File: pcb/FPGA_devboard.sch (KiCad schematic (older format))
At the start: 2 parts, among them X3 AC7020, X4 Conn_02x05_Odd_Even

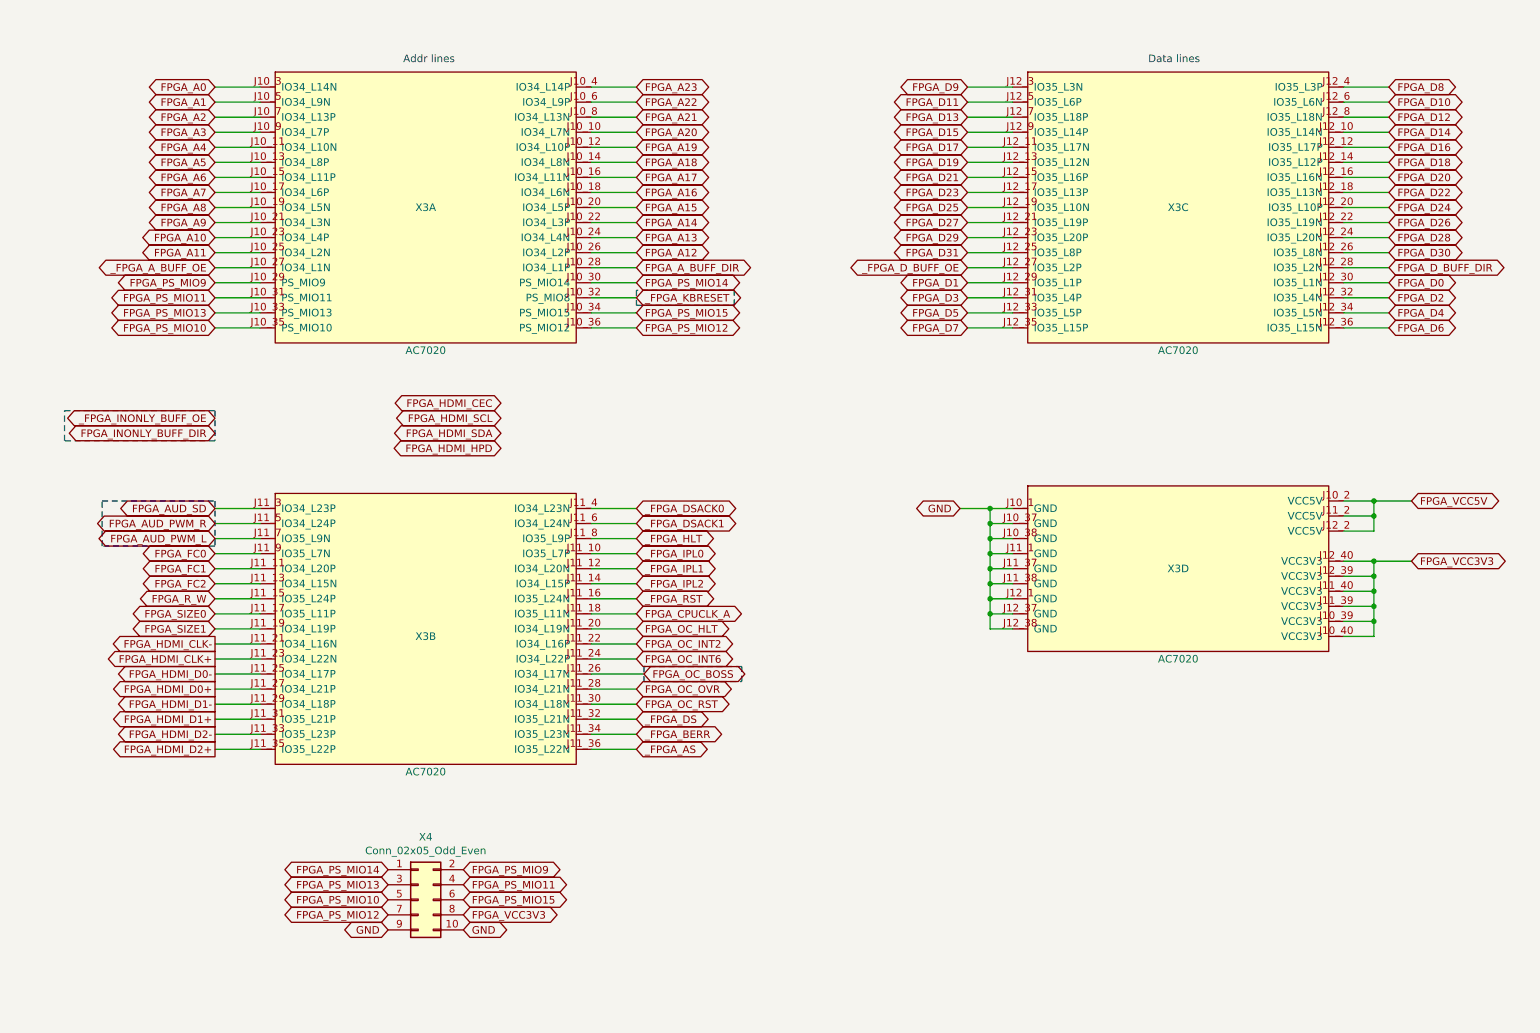
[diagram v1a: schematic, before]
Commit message: time to stop for today
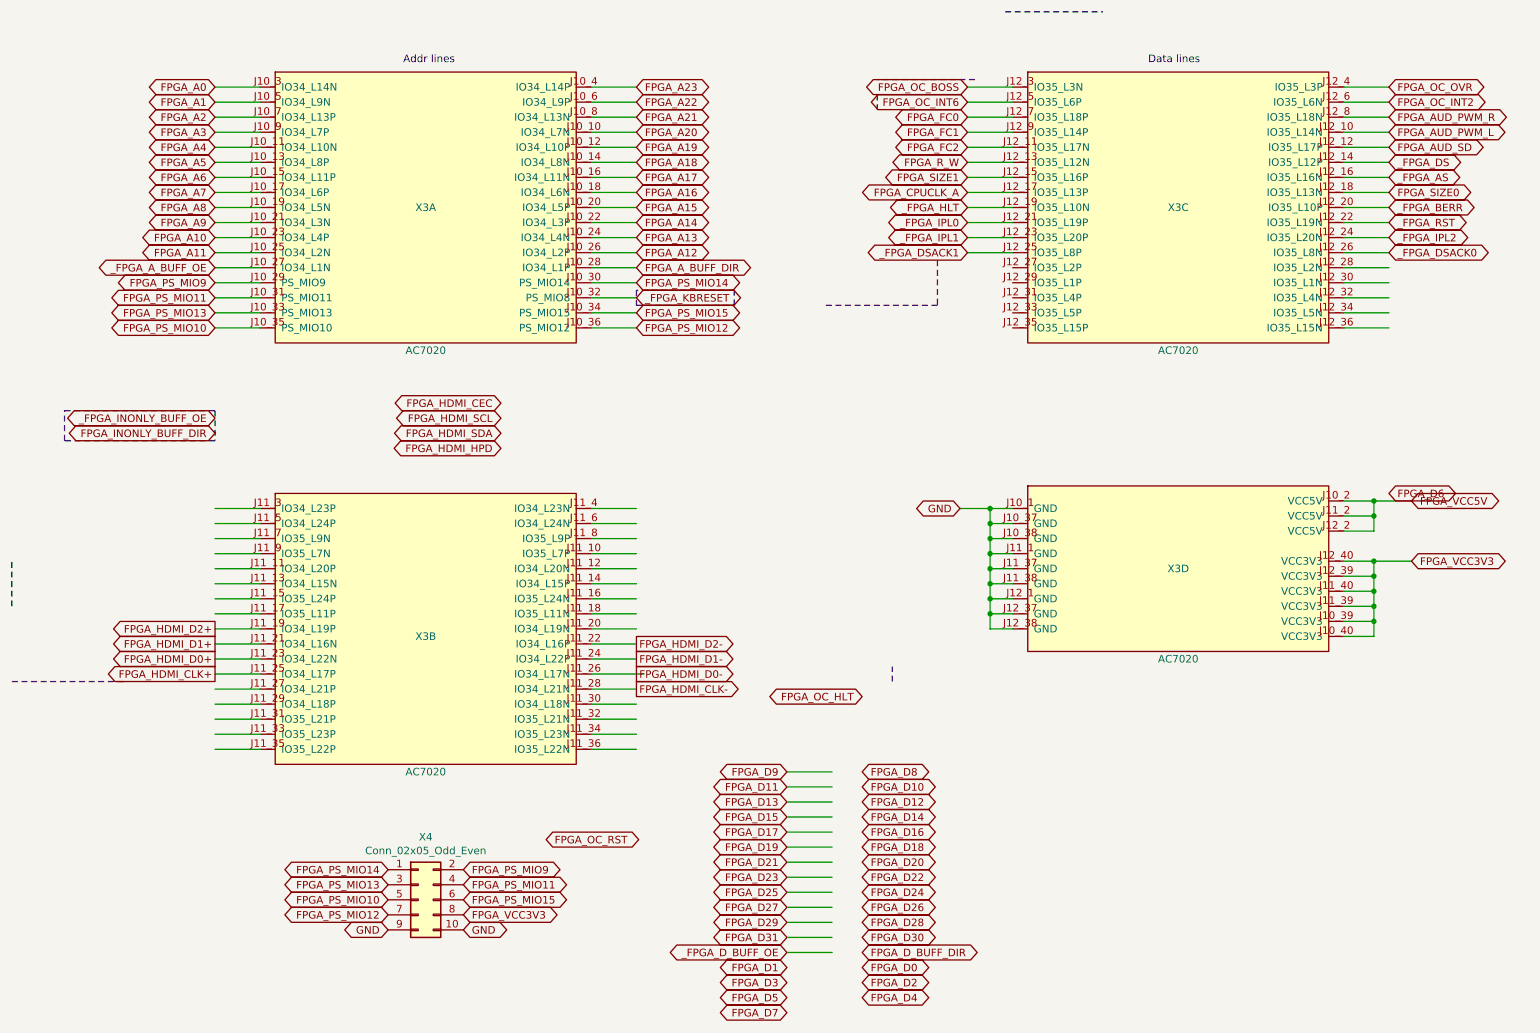
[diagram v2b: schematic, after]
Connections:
- wire segments 138 -> 146
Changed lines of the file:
@@
 	4300 6000 4600 6000
 Wire Wire Line
-	6800 3200 7100 3200
-Wire Wire Line
-	6800 1600 7100 1600
-Wire Wire Line
-	6800 1700 7100 1700
+	5600 7350 5900 7350
 Wire Wire Line
 	6800 1800 7100 1800
@@
 	6800 2100 7100 2100
 Wire Wire Line
-	6800 2200 7100 2200
-Wire Wire Line
-	6800 2300 7100 2300
-Wire Wire Line
-	6800 2400 7100 2400
-Wire Wire Line
-	6800 2500 7100 2500
-Wire Wire Line
-	6800 2600 7100 2600
-Wire Wire Line
-	6800 2700 7100 2700
-Wire Wire Line
-	6800 2800 7100 2800
-Wire Wire Line
-	6800 2900 7100 2900
-Wire Wire Line
-	6800 3000 7100 3000
-Wire Wire Line
-	6800 3100 7100 3100
+	5600 6150 5900 6150
+Wire Wire Line
+	5600 6250 5900 6250
+Wire Wire Line
+	5600 6350 5900 6350
+Wire Wire Line
+	5600 6450 5900 6450
+Wire Wire Line
+	5600 6550 5900 6550
+Wire Wire Line
+	5600 6650 5900 6650
+Wire Wire Line
+	5600 6750 5900 6750
+Wire Wire Line
+	5600 6850 5900 6850
+Wire Wire Line
+	5600 6950 5900 6950
+Wire Wire Line
+	5600 7050 5900 7050
+Wire Wire Line
+	5600 7150 5900 7150
+Wire Wire Line
+	5600 7250 5900 7250
 Wire Wire Line
 	9300 1600 9600 1600
@@
 Text GLabel 1800 2800 0    50   BiDi ~ 0
 _FPGA_A_BUFF_OE
-Text GLabel 9600 2900 2    50   BiDi ~ 0
+Text GLabel 6100 7450 2    50   BiDi ~ 0
 FPGA_D0
-Text GLabel 6800 2900 0    50   BiDi ~ 0
+Text GLabel 5600 7450 0    50   BiDi ~ 0
 FPGA_D1
-Text GLabel 9600 3000 2    50   BiDi ~ 0
+Text GLabel 6100 7550 2    50   BiDi ~ 0
 FPGA_D2
-Text GLabel 6800 3000 0    50   BiDi ~ 0
+Text GLabel 5600 7550 0    50   BiDi ~ 0
 FPGA_D3
-Text GLabel 9600 3100 2    50   BiDi ~ 0
+Text GLabel 6100 7650 2    50   BiDi ~ 0
 FPGA_D4
-Text GLabel 6800 3100 0    50   BiDi ~ 0
+Text GLabel 5600 7650 0    50   BiDi ~ 0
 FPGA_D5
-Text GLabel 9600 3200 2    50   BiDi ~ 0
+Text GLabel 9600 4300 2    50   BiDi ~ 0
 FPGA_D6
-Text GLabel 6800 3200 0    50   BiDi ~ 0
+Text GLabel 5600 7750 0    50   BiDi ~ 0
 FPGA_D7
-Text GLabel 9600 1600 2    50   BiDi ~ 0
+Text GLabel 6100 6150 2    50   BiDi ~ 0
 FPGA_D8
-Text GLabel 6800 1600 0    50   BiDi ~ 0
+Text GLabel 5600 6150 0    50   BiDi ~ 0
 FPGA_D9
-Text GLabel 9600 1700 2    50   BiDi ~ 0
+Text GLabel 6100 6250 2    50   BiDi ~ 0
 FPGA_D10
-Text GLabel 6800 1700 0    50   BiDi ~ 0
+Text GLabel 5600 6250 0    50   BiDi ~ 0
 FPGA_D11
+Text GLabel 6100 6350 2    50   BiDi ~ 0
+FPGA_D12
+Text GLabel 5600 6350 0    50   BiDi ~ 0
+FPGA_D13
+Text GLabel 6100 6450 2    50   BiDi ~ 0
+FPGA_D14
+Text GLabel 5600 6450 0    50   BiDi ~ 0
+FPGA_D15
+Text GLabel 6100 6550 2    50   BiDi ~ 0
+FPGA_D16
+Text GLabel 5600 6550 0    50   BiDi ~ 0
+FPGA_D17
+Text GLabel 6100 6650 2    50   BiDi ~ 0
+FPGA_D18
+Text GLabel 5600 6650 0    50   BiDi ~ 0
+FPGA_D19
+Text GLabel 6100 6750 2    50   BiDi ~ 0
+FPGA_D20
+Text GLabel 5600 6750 0    50   BiDi ~ 0
+FPGA_D21
+Text GLabel 6100 6850 2    50   BiDi ~ 0
+FPGA_D22
+Text GLabel 5600 6850 0    50   BiDi ~ 0
+FPGA_D23
+Text GLabel 6100 6950 2    50   BiDi ~ 0
+FPGA_D24
+Text GLabel 5600 6950 0    50   BiDi ~ 0
+FPGA_D25
+Text GLabel 6100 7050 2    50   BiDi ~ 0
+FPGA_D26
+Text GLabel 5600 7050 0    50   BiDi ~ 0
+FPGA_D27
+Text GLabel 6100 7150 2    50   BiDi ~ 0
+FPGA_D28
+Text GLabel 5600 7150 0    50   BiDi ~ 0
+FPGA_D29
+Text GLabel 6100 7250 2    50   BiDi ~ 0
+FPGA_D30
+Text GLabel 5600 7250 0    50   BiDi ~ 0
+FPGA_D31
+Text GLabel 6100 7350 2    50   BiDi ~ 0
+FPGA_D_BUFF_DIR
+Text GLabel 5600 7350 0    50   BiDi ~ 0
+_FPGA_D_BUFF_OE
+Text GLabel 9600 1900 2    50   BiDi ~ 0
+FPGA_AUD_PWM_L
 Text GLabel 9600 1800 2    50   BiDi ~ 0
-FPGA_D12
-Text GLabel 6800 1800 0    50   BiDi ~ 0
-FPGA_D13
-Text GLabel 9600 1900 2    50   BiDi ~ 0
-FPGA_D14
-Text GLabel 6800 1900 0    50   BiDi ~ 0
-FPGA_D15
+FPGA_AUD_PWM_R
 Text GLabel 9600 2000 2    50   BiDi ~ 0
-FPGA_D16
-Text GLabel 6800 2000 0    50   BiDi ~ 0
-FPGA_D17
-Text GLabel 9600 2100 2    50   BiDi ~ 0
-FPGA_D18
-Text GLabel 6800 2100 0    50   BiDi ~ 0
-FPGA_D19
-Text GLabel 9600 2200 2    50   BiDi ~ 0
-FPGA_D20
-Text GLabel 6800 2200 0    50   BiDi ~ 0
-FPGA_D21
-Text GLabel 9600 2300 2    50   BiDi ~ 0
-FPGA_D22
-Text GLabel 6800 2300 0    50   BiDi ~ 0
-FPGA_D23
-Text GLabel 9600 2400 2    50   BiDi ~ 0
-FPGA_D24
-Text GLabel 6800 2400 0    50   BiDi ~ 0
-FPGA_D25
-Text GLabel 9600 2500 2    50   BiDi ~ 0
-FPGA_D26
-Text GLabel 6800 2500 0    50   BiDi ~ 0
-FPGA_D27
-Text GLabel 9600 2600 2    50   BiDi ~ 0
-FPGA_D28
-Text GLabel 6800 2600 0    50   BiDi ~ 0
-FPGA_D29
-Text GLabel 9600 2700 2    50   BiDi ~ 0
-FPGA_D30
-Text GLabel 6800 2700 0    50   BiDi ~ 0
-FPGA_D31
-Text GLabel 9600 2800 2    50   BiDi ~ 0
-FPGA_D_BUFF_DIR
-Text GLabel 6800 2800 0    50   BiDi ~ 0
-_FPGA_D_BUFF_OE
-Text GLabel 1800 4600 0    50   BiDi ~ 0
-FPGA_AUD_PWM_L
-Text GLabel 1800 4500 0    50   BiDi ~ 0
-FPGA_AUD_PWM_R
-Text GLabel 1800 4400 0    50   BiDi ~ 0
 FPGA_AUD_SD
-Text GLabel 4650 5500 2    50   BiDi ~ 0
-FPGA_OC_BOSS
-Text GLabel 4600 5200 2    50   BiDi ~ 0
-FPGA_OC_HLT
-Text GLabel 4600 5400 2    50   BiDi ~ 0
-FPGA_OC_INT6
-Text GLabel 4600 5600 2    50   BiDi ~ 0
-FPGA_OC_OVR
-Text GLabel 4600 5700 2    50   BiDi ~ 0
+Text GLabel 4000 6600 2    50   BiDi ~ 0
 FPGA_OC_RST
-Text GLabel 4600 4400 2    50   BiDi ~ 0
-_FPGA_DSACK0
-Text GLabel 4600 4500 2    50   BiDi ~ 0
-_FPGA_DSACK1
-Text GLabel 4600 4600 2    50   BiDi ~ 0
-_FPGA_HLT
-Text GLabel 4600 4700 2    50   BiDi ~ 0
-_FPGA_IPL0
-Text GLabel 4600 4800 2    50   BiDi ~ 0
-_FPGA_IPL1
-Text GLabel 4600 4900 2    50   BiDi ~ 0
-_FPGA_IPL2
-Text GLabel 4600 5000 2    50   BiDi ~ 0
-_FPGA_RST
 Text GLabel 2950 7200 0    50   BiDi ~ 0
 GND
@@
 	4600 3200 4300 3200
 Wire Notes Line
-	1050 4650 1050 4350
-Wire Notes Line
-	1050 4350 1800 4350
-Wire Notes Line
-	1800 4650 1050 4650
-Wire Notes Line
-	5300 5450 4650 5450
-Wire Notes Line
-	4650 5450 4650 5550
-Wire Notes Line
-	4650 5550 5300 5550
-Wire Notes Line
-	5300 5550 5300 5450
+	450  5050 450  4750
+Wire Notes Line
+	450  5550 1200 5550
+Wire Notes Line
+	6600 3050 5850 3050
+Wire Notes Line
+	6200 1650 6200 1750
 Wire Notes Line
 	1800 3750 1800 3950
@@
 Wire Notes Line
 	4600 3050 5250 3050
-Text GLabel 1800 6000 0    50   Output ~ 0
+Text GLabel 1800 5200 0    50   Output ~ 0
 FPGA_HDMI_D2+
-Text GLabel 1800 5900 0    50   Output ~ 0
+Text GLabel 4600 5300 2    50   Output ~ 0
 FPGA_HDMI_D2-
-Text GLabel 1800 5800 0    50   Output ~ 0
+Text GLabel 1800 5300 0    50   Output ~ 0
 FPGA_HDMI_D1+
-Text GLabel 1800 5600 0    50   Output ~ 0
+Text GLabel 1800 5400 0    50   Output ~ 0
 FPGA_HDMI_D0+
+Text GLabel 4600 5500 2    50   Output ~ 0
+FPGA_HDMI_D0-
+Text GLabel 4600 5400 2    50   Output ~ 0
+FPGA_HDMI_D1-
 Text GLabel 1800 5500 0    50   Output ~ 0
-FPGA_HDMI_D0-
-Text GLabel 1800 5700 0    50   Output ~ 0
-FPGA_HDMI_D1-
-Text GLabel 1800 5400 0    50   Output ~ 0
 FPGA_HDMI_CLK+
 Wire Notes Line
@@
 Wire Notes Line
 	800  3750 1800 3750
-Text GLabel 4600 5800 2    50   BiDi ~ 0
-_FPGA_DS
-Text GLabel 4600 5900 2    50   BiDi ~ 0
-_FPGA_BERR
-Text GLabel 4600 6000 2    50   BiDi ~ 0
+Text GLabel 9600 2200 2    50   BiDi ~ 0
 _FPGA_AS
-Text GLabel 1800 5200 0    50   BiDi ~ 0
+Text GLabel 6800 2200 0    50   BiDi ~ 0
 FPGA_SIZE1
-Text GLabel 1800 5100 0    50   BiDi ~ 0
+Text GLabel 9600 2300 2    50   BiDi ~ 0
 FPGA_SIZE0
-Text GLabel 1800 5000 0    50   BiDi ~ 0
-FPGA_R_W
-Text GLabel 1800 4900 0    50   BiDi ~ 0
-FPGA_FC2
-Text GLabel 1800 4800 0    50   BiDi ~ 0
-FPGA_FC1
-Text GLabel 1800 4700 0    50   BiDi ~ 0
-FPGA_FC0
-Text GLabel 4600 5100 2    50   BiDi ~ 0
-FPGA_CPUCLK_A
 Text GLabel 1800 3900 0    50   BiDi ~ 0
 FPGA_INONLY_BUFF_DIR
@@
 _FPGA_INONLY_BUFF_OE
 Wire Notes Line
-	1800 4350 1800 4650
-Text GLabel 1800 5300 0    50   Output ~ 0
+	6600 2750 6600 3050
+Text GLabel 4600 5600 2    50   Output ~ 0
 FPGA_HDMI_CLK-
 Wire Wire Line
@@
 Text GLabel 3700 4000 0    50   BiDi ~ 0
 FPGA_HDMI_HPD
-Text GLabel 4600 5300 2    50   BiDi ~ 0
-FPGA_OC_INT2
 Wire Wire Line
 	4300 5500 4650 5500
@@
 Wire Notes Line
 	5250 3050 5250 2950
+Text GLabel 9600 1700 2    50   BiDi ~ 0
+FPGA_OC_INT2
+Wire Notes Line
+	6300 5550 6300 5450
+Wire Notes Line
+	7050 1100 7700 1100
+Wire Notes Line
+	6850 1550 6200 1550
+Text GLabel 6800 2600 0    50   BiDi ~ 0
+_FPGA_IPL1
+Text GLabel 6800 2500 0    50   BiDi ~ 0
+_FPGA_IPL0
+Text GLabel 6800 2400 0    50   BiDi ~ 0
+_FPGA_HLT
+Text GLabel 6800 2700 0    50   BiDi ~ 0
+_FPGA_DSACK1
+Text GLabel 9600 1600 2    50   BiDi ~ 0
+FPGA_OC_OVR
+Text GLabel 6800 1700 0    50   BiDi ~ 0
+FPGA_OC_INT6
+Text GLabel 6100 5650 0    50   BiDi ~ 0
+FPGA_OC_HLT
+Text GLabel 6800 1600 0    50   BiDi ~ 0
+FPGA_OC_BOSS
+Text GLabel 6800 2100 0    50   BiDi ~ 0
+FPGA_R_W
+Text GLabel 6800 1800 0    50   BiDi ~ 0
+FPGA_FC0
+Text GLabel 6800 1900 0    50   BiDi ~ 0
+FPGA_FC1
+Text GLabel 6800 2000 0    50   BiDi ~ 0
+FPGA_FC2
+Text GLabel 9600 2100 2    50   BiDi ~ 0
+_FPGA_DS
+Wire Wire Line
+	6800 2200 7100 2200
+Wire Wire Line
+	7100 2300 6800 2300
+Wire Wire Line
+	6800 2400 7100 2400
+Wire Wire Line
+	7100 2500 6800 2500
+Wire Wire Line
+	6800 2600 7100 2600
+Wire Wire Line
+	7100 1600 6800 1600
+Wire Wire Line
+	6800 1700 7100 1700
+Wire Wire Line
+	7100 2700 6800 2700
+Text GLabel 9600 2700 2    50   BiDi ~ 0
+_FPGA_DSACK0
+Text GLabel 9600 2600 2    50   BiDi ~ 0
+_FPGA_IPL2
+Text GLabel 9600 2500 2    50   BiDi ~ 0
+_FPGA_RST
+Text GLabel 9600 2400 2    50   BiDi ~ 0
+_FPGA_BERR
+Text GLabel 6800 2300 0    50   BiDi ~ 0
+FPGA_CPUCLK_A
 $EndSCHEMATC
